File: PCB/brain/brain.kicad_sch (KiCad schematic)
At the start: 221 parts, among them J1 Screw_Terminal_01x02, J10 Conn_01x12, J11 Conn_01x04, J12 BAT, J2 Conn_01x04, J3 RJ45_Hanrun_HR911105A_Horizon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, J4 Conn_01x04, J5 Conn_01x04, J6 Conn_01x04, J7 Conn_01x06, J8 Conn_01x06, J9 Motor, Q1 CSD17577Q3A, Q2 CSD17577Q3A, U1 ESP32-S3-WROOM-1, U10 MAX17049G+T10, U11 AP64501SP-13, U12 AP63205WU, U14 AP63203WU, U2 TMC2209-LA, U3 W5500, U4 MAX98357A, U5 TPD2E2U06DCK, U7 R5460N214AF-TR-FE, U8 CH221K, U9 BQ25792, Y1 25MHz

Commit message: more pcb
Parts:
- J10: footprint Connector_PinSocket_2.54mm:PinSocket_1x12_P2.54mm_Vertical -> Connector_PinHeader_2.54mm:PinHeader_2x06_P2.54mm_Vertical
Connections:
- net EN: no longer J10.10 (Pin_10), R46.1, U1.11 (IO18), U2.2 (~{EN})
- new net TmcEN: J10.10 (Pin_10), R46.1, U1.11 (IO18), U2.2 (~{EN})
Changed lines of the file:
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@@
 		)
 	)
+	(global_label "TmcEN"
+		(shape input)
+		(at 461.01 331.47 180)
+		(fields_autoplaced yes)
+		(effects
+			(font
+				(size 1.27 1.27)
+			)
+			(justify right)
+		)
+		(property "Intersheetrefs" "${INTERSHEET_REFS}"
+			(at 451.7958 331.47 0)
+			(hide yes)
+			(show_name no)
+			(do_not_autoplace no)
+			(effects
+				(font
+					(size 1.27 1.27)
+				)
+				(justify right)
+			)
+		)
+	)
 	(global_label "PMODE0"
 		(shape input)
@@
 		)
 	)
-	(global_label "EN"
-		(shape input)
-		(at 397.51 377.19 180)
-		(fields_autoplaced yes)
-		(effects
-			(font
-				(size 1.27 1.27)
-			)
-			(justify right)
-		)
-		(property "Intersheetrefs" "${INTERSHEET_REFS}"
-			(at 392.0453 377.19 0)
-			(hide yes)
-			(show_name no)
-			(do_not_autoplace no)
-			(effects
-				(font
-					(size 1.27 1.27)
-				)
-				(justify right)
-			)
-		)
-	)
 	(global_label "RSTn"
 		(shape input)
@@
 		)
 	)
+	(global_label "TmcEN"
+		(shape input)
+		(at 375.92 377.19 0)
+		(fields_autoplaced yes)
+		(effects
+			(font
+				(size 1.27 1.27)
+			)
+			(justify left)
+		)
+		(property "Intersheetrefs" "${INTERSHEET_REFS}"
+			(at 385.1342 377.19 0)
+			(hide yes)
+			(show_name no)
+			(do_not_autoplace no)
+			(effects
+				(font
+					(size 1.27 1.27)
+				)
+				(justify left)
+			)
+		)
+	)
 	(global_label "D+"
 		(shape input)
@@
 		)
 	)
-	(global_label "EN"
+	(global_label "TmcEN"
 		(shape input)
-		(at 375.92 377.19 0)
+		(at 397.51 377.19 180)
 		(fields_autoplaced yes)
 		(effects
@@
 				(size 1.27 1.27)
 			)
-			(justify left)
+			(justify right)
 		)
 		(property "Intersheetrefs" "${INTERSHEET_REFS}"
-			(at 381.3847 377.19 0)
+			(at 388.2958 377.19 0)
 			(hide yes)
 			(show_name no)
@@
 					(size 1.27 1.27)
 				)
-				(justify left)
+				(justify right)
 			)
 		)
@@
 		)
 	)
-	(global_label "EN"
+	(global_label "TmcEN"
 		(shape input)
 		(at 101.6 58.42 0)
@@
 		)
 		(property "Intersheetrefs" "${INTERSHEET_REFS}"
-			(at 107.0647 58.42 0)
+			(at 110.8142 58.42 0)
 			(hide yes)
 			(show_name no)
@@
 		)
 	)
-	(global_label "EN"
-		(shape input)
-		(at 461.01 331.47 180)
-		(fields_autoplaced yes)
-		(effects
-			(font
-				(size 1.27 1.27)
-			)
-			(justify right)
-		)
-		(property "Intersheetrefs" "${INTERSHEET_REFS}"
-			(at 455.5453 331.47 0)
-			(hide yes)
-			(show_name no)
-			(do_not_autoplace no)
-			(effects
-				(font
-					(size 1.27 1.27)
-				)
-				(justify right)
-			)
-		)
-	)
 	(global_label "DIAG"
 		(shape input)
@@
 		(property "LCSC Part" "C77020"
 			(at 0 629.92 0)
+			(hide yes)
 			(show_name no)
 			(do_not_autoplace no)
@@
 		(property "LCSC Part" "C77020"
 			(at 0 662.94 0)
+			(hide yes)
 			(show_name no)
 			(do_not_autoplace no)
@@
 			)
 		)
-		(property "Footprint" "Connector_PinSocket_2.54mm:PinSocket_1x12_P2.54mm_Vertical"
+		(property "Footprint" "Connector_PinHeader_2.54mm:PinHeader_2x06_P2.54mm_Vertical"
 			(at 466.09 321.31 0)
 			(hide yes)

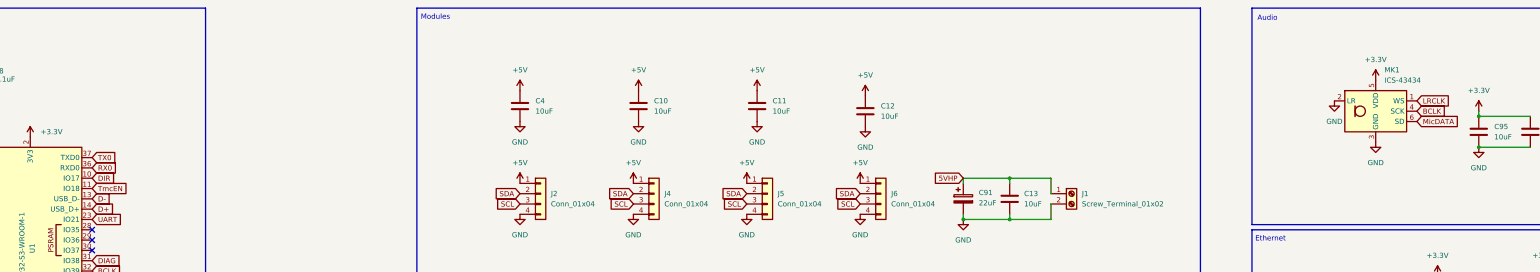
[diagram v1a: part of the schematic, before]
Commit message: moar pcb
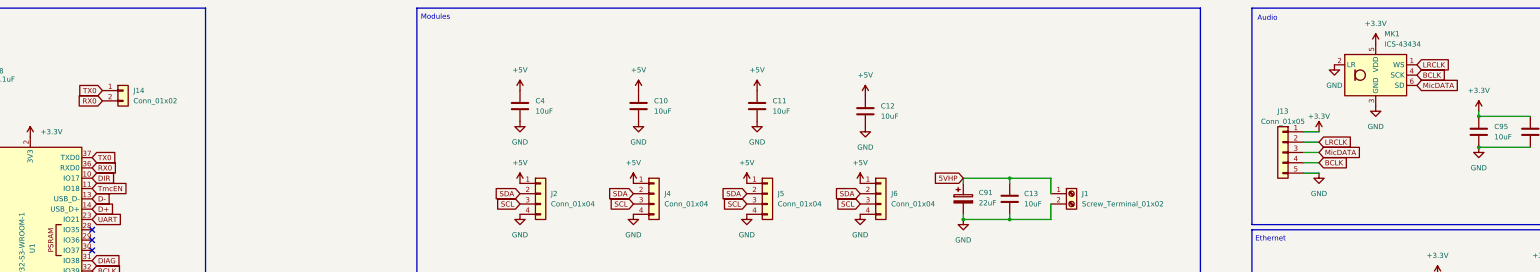
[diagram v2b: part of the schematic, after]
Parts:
- added J13: Conn_01x05, Connector_JST:JST_XH_B5B-XH-A_1x05_P2.50mm_Vertical, symbol Connector_Generic:Conn_01x05
- added J14: Conn_01x02, Connector_PinSocket_2.54mm:PinSocket_1x02_P2.54mm_Vertical, symbol Connector_Generic:Conn_01x02
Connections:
- net +3.3V: now also J13.1 (Pin_1)
- net BCLK: now also J13.4 (Pin_4)
- net GND: now also J13.5 (Pin_5)
- net LRCLK: now also J13.2 (Pin_2)
- net MicDATA: now also J13.3 (Pin_3)
- net RX0: now also J14.2 (Pin_2)
- net TX0: now also J14.1 (Pin_1)
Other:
- moved on the sheet: MK1

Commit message: more pcb
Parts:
- U1: footprint RF_Module:ESP32-S3-WROOM-1 -> RF_Module:ESP32-S3-WROOM-1U
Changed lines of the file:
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@@
 			)
 		)
-		(property "Footprint" "RF_Module:ESP32-S3-WROOM-1"
+		(property "Footprint" "RF_Module:ESP32-S3-WROOM-1U"
 			(at 86.36 71.12 0)
 			(hide yes)
